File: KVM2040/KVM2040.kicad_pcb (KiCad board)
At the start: 2 copper layers, 30 x 20 mm, 3 parts, among them J1 HDMI_A_1.4, U1 RP2040, U2 TS3DV642A0RUAR

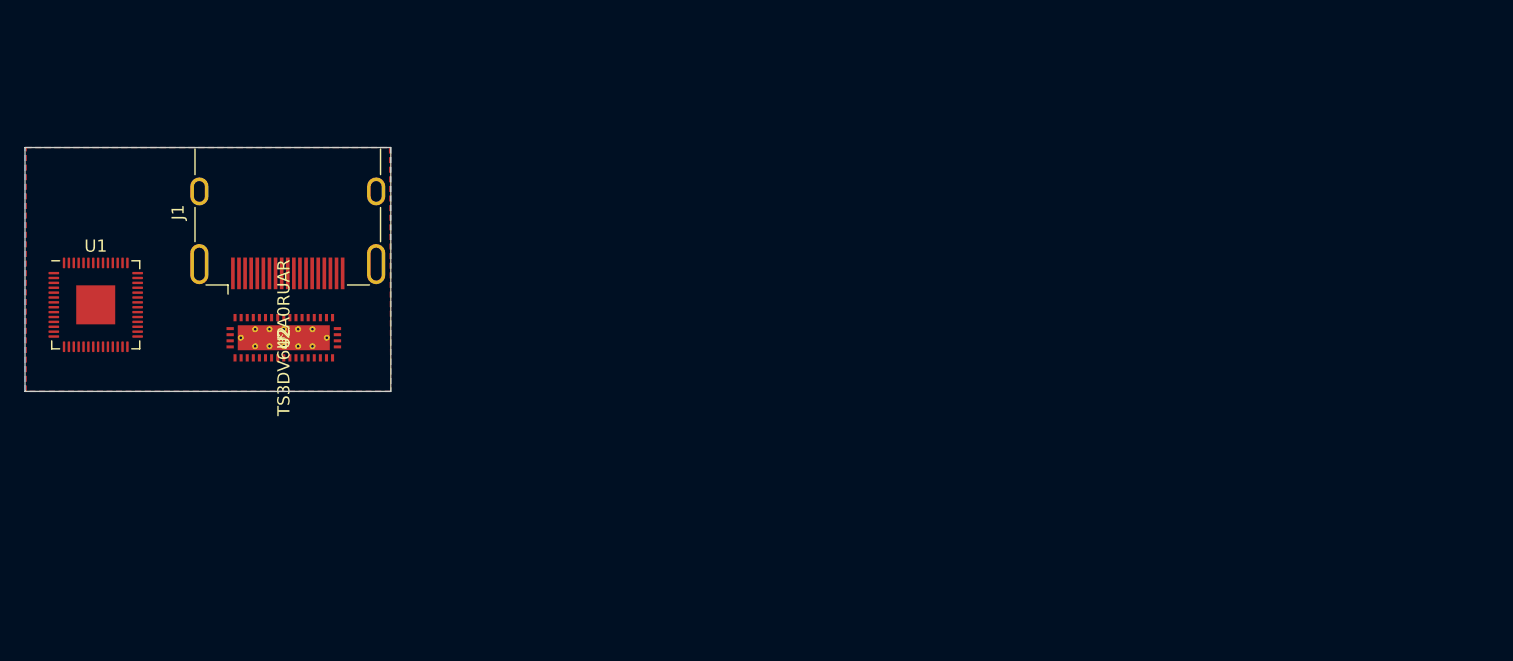
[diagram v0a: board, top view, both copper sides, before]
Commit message: USB progress
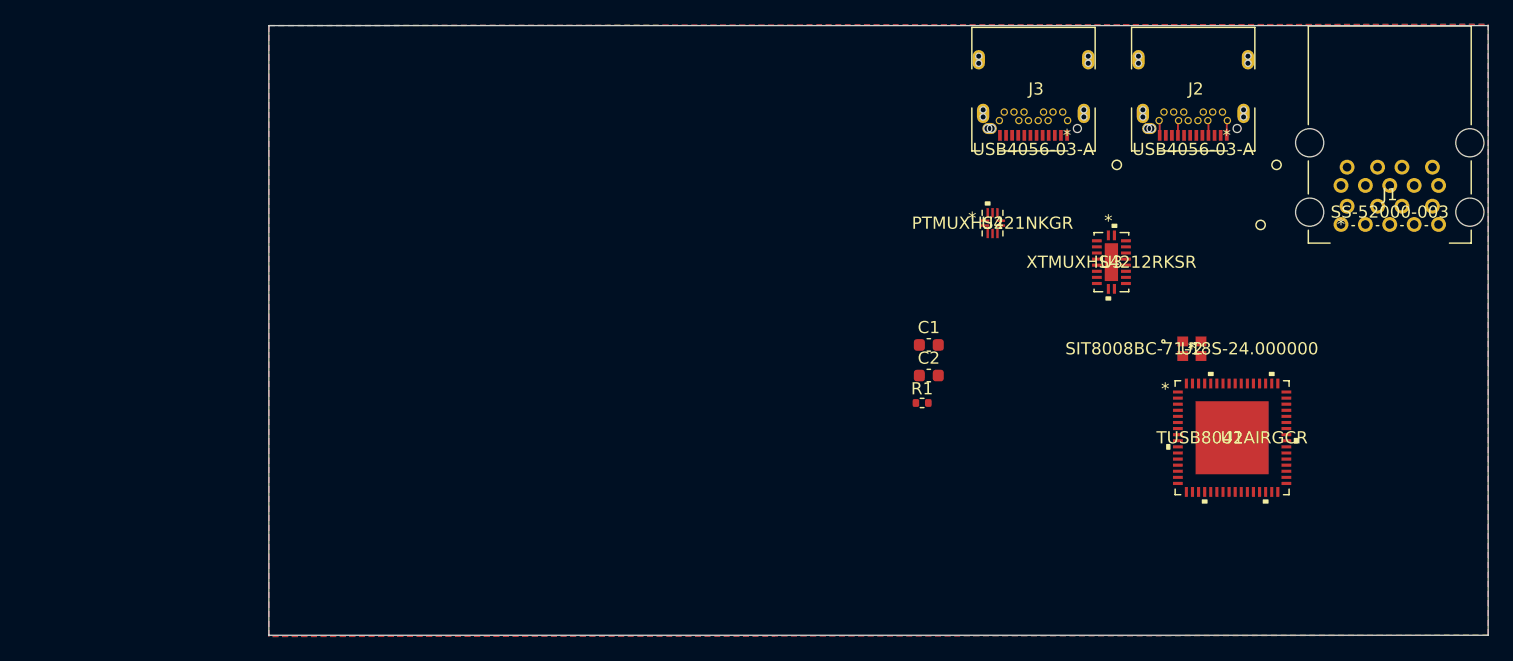
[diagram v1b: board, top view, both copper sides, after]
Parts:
- added C1: 0.1uF, Capacitor_SMD:C_0603_1608Metric, F.Cu at (204.1, 76.2)
- added C2: 0.001uF, Capacitor_SMD:C_0603_1608Metric, F.Cu at (204.1, 78.7)
- added J2: USB4056-03-A, USB4056:USB4056-03-A, F.Cu at (228.6, 59.0)
- added J3: USB4056-03-A, USB4056:USB4056-03-A, F.Cu at (215.5, 59.0)
- added R1: 1M, Resistor_SMD:R_0402_1005Metric, F.Cu at (203.6, 81.0)
- added U3: XTMUXHS4212RKSR, TMUXHS4212:XTMUXHS4212RKSR, F.Cu at (219.1, 69.4)
- added U4: PTMUXHS221NKGR, TMUXHS221:PTMUXHS221NKGR, F.Cu at (209.4, 66.2)
- J1: value HDMI_A_1.4 -> SS-52000-003; footprint Connector_HDMI:HDMI_A_Molex_208658-1001_Horizontal -> SS-52000:SS-52000-003
- U1: value RP2040 -> TUSB8042AIRGCR; footprint Package_DFN_QFN:QFN-56-1EP_7x7mm_P0.4mm_EP3.2x3.2mm -> TUSB8042A:TUSB8042AIRGCR
- U2: value TS3DV642A0RUAR -> SIT8008BC-71-18S-24.000000; footprint TS3DV642:TS3DV642A0RUAR -> SIT8008BC:SIT8008BC-71-18S-24.000000
- moved U1 93.8 mm to (229.0, 83.8)
- moved J1 86.4 mm to (237.9, 66.3), turned to 180 degrees
- moved U2 74.5 mm to (225.7, 76.5), turned to 0 degrees
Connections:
- J1 pad 1: /D2+ -> GND
- J1 pad 10: /CK+ -> unconnected-(J1-Pad10)
- J1 pad 12: /CK- -> unconnected-(J1-Pad12)
- J1 pad 13: /CEC -> unconnected-(J1-Pad13)
- J1 pad 14: /UTILITY -> +5V
- J1 pad 15: /SCL -> unconnected-(J1-Pad15)
- J1 pad 16: /SDA -> unconnected-(J1-Pad16)
- J1 pad 18: +5V -> unconnected-(J1-Pad18)
- J1 pad 2: GND -> unconnected-(J1-Pad2)
- J1 pad 3: /D2- -> unconnected-(J1-Pad3)
- J1 pad 4: /D1+ -> +5V
- J1 pad 5: GND -> unconnected-(J1-Pad5)
- J1 pad 6: /D1- -> unconnected-(J1-Pad6)
- J1 pad 7: /D0+ -> GND
- J1 pad 8: GND -> unconnected-(J1-Pad8)
- U1 pad 1: Net-(U1-IOVDD-Pad1) -> unconnected-(U1-USB_DP_DN1-Pad1)
- U1 pad 10: Net-(U1-IOVDD-Pad1) -> unconnected-(U1-USB_DM_DN2-Pad10)
- U1 pad 2: /EN -> unconnected-(U1-USB_DM_DN1-Pad2)
- U1 pad 22: Net-(U1-IOVDD-Pad1) -> unconnected-(U1-USB_SSRXP_DN3-Pad22)
- U1 pad 23: Net-(U1-DVDD-Pad23) -> unconnected-(U1-USB_SSRXM_DN3-Pad23)
- U1 pad 3: /SEL1 -> unconnected-(U1-USB_SSTXP_DN1-Pad3)
- U1 pad 33: Net-(U1-IOVDD-Pad1) -> unconnected-(U1-PWRCTL3/BATEM/-Pad33)
- U1 pad 4: /SEL2 -> unconnected-(U1-USB_SSTXM_DN1-Pad4)
- U1 pad 42: Net-(U1-IOVDD-Pad1) -> unconnected-(U1-GANGED/SMBA2/HS_UP-Pad42)
- U1 pad 48: unconnected-(U1-USB_VDD-Pad48) -> VBUS
- U1 pad 49: Net-(U1-IOVDD-Pad1) -> unconnected-(U1-TEST-Pad49)
- U1 pad 50: Net-(U1-DVDD-Pad23) -> unconnected-(U1-GRSTz-Pad50)
- U2 pad 1: +5V -> unconnected-(U2-OE/ST/NC-Pad1)
- U2 pad 2: /EN -> GND
- U2 pad 3: /SCL -> /USB_Switch/XI
- U2 pad 4: /SDA -> +3.3V
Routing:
- net VBUS: track 0.00 -> 2.47 mm
- net GND: track 0.00 -> 2.47 mm
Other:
- board size 30 x 20 mm -> 100 x 50 mm
